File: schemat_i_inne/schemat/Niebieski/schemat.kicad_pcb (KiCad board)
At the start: 2 copper layers, 195.6 x 86.4 mm, 34 parts, among them J1 Hole1, J2 Hole2, J3 Hole3, J4 Hole4, J5 RJ45, J6 Conn_01x01_Male, J7 Conn_01x01_Male, SW1 SW_DIP_x01, SW2 Left, SW3 Up, SW4 Down, SW5 Right, SW6 Jump, SW7 Punch, U1 ATmega32A-AU, U2 L7805, U3 WG12864B-STBL, U4 LF33_TO252, U5 SN74LS07, U6 SD, Y1 16Mhz

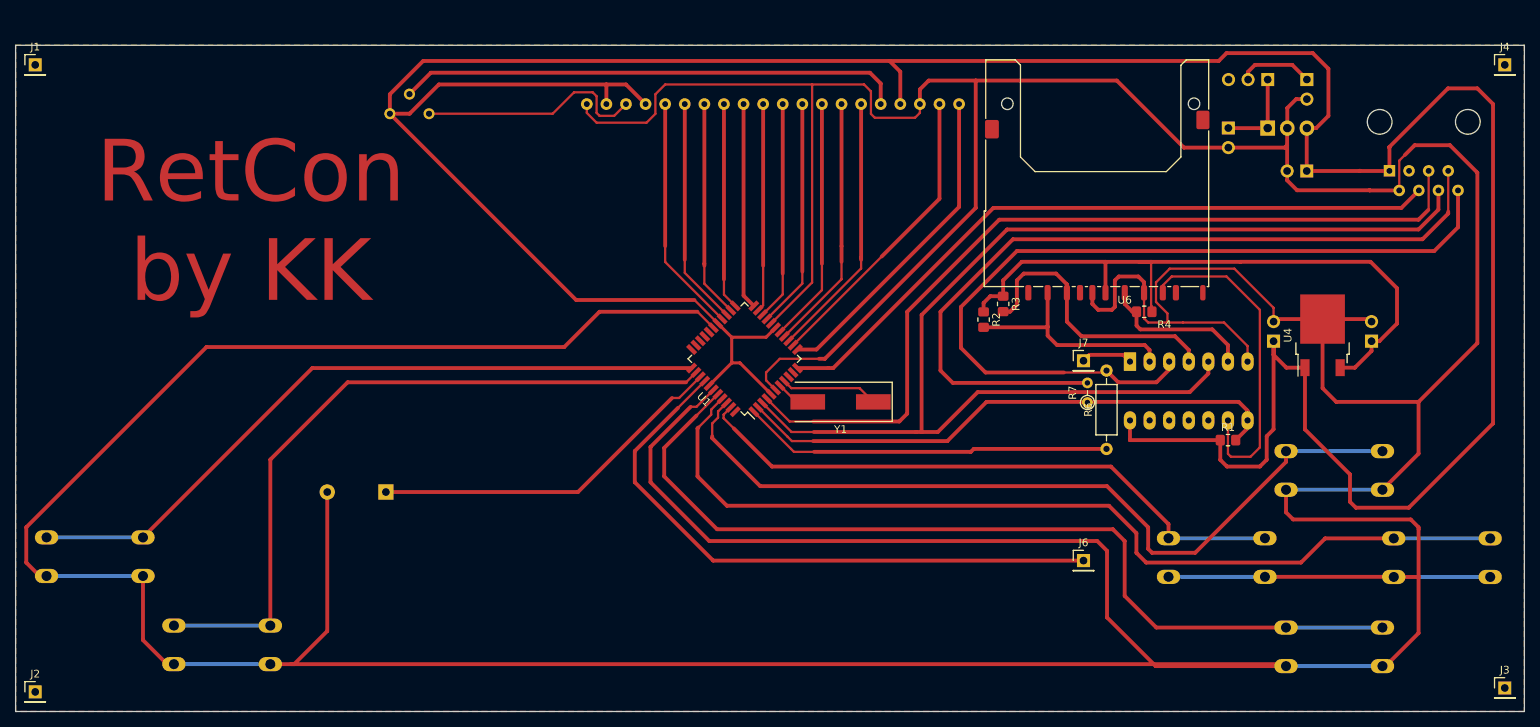
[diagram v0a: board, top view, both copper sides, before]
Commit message: new version of schema and board
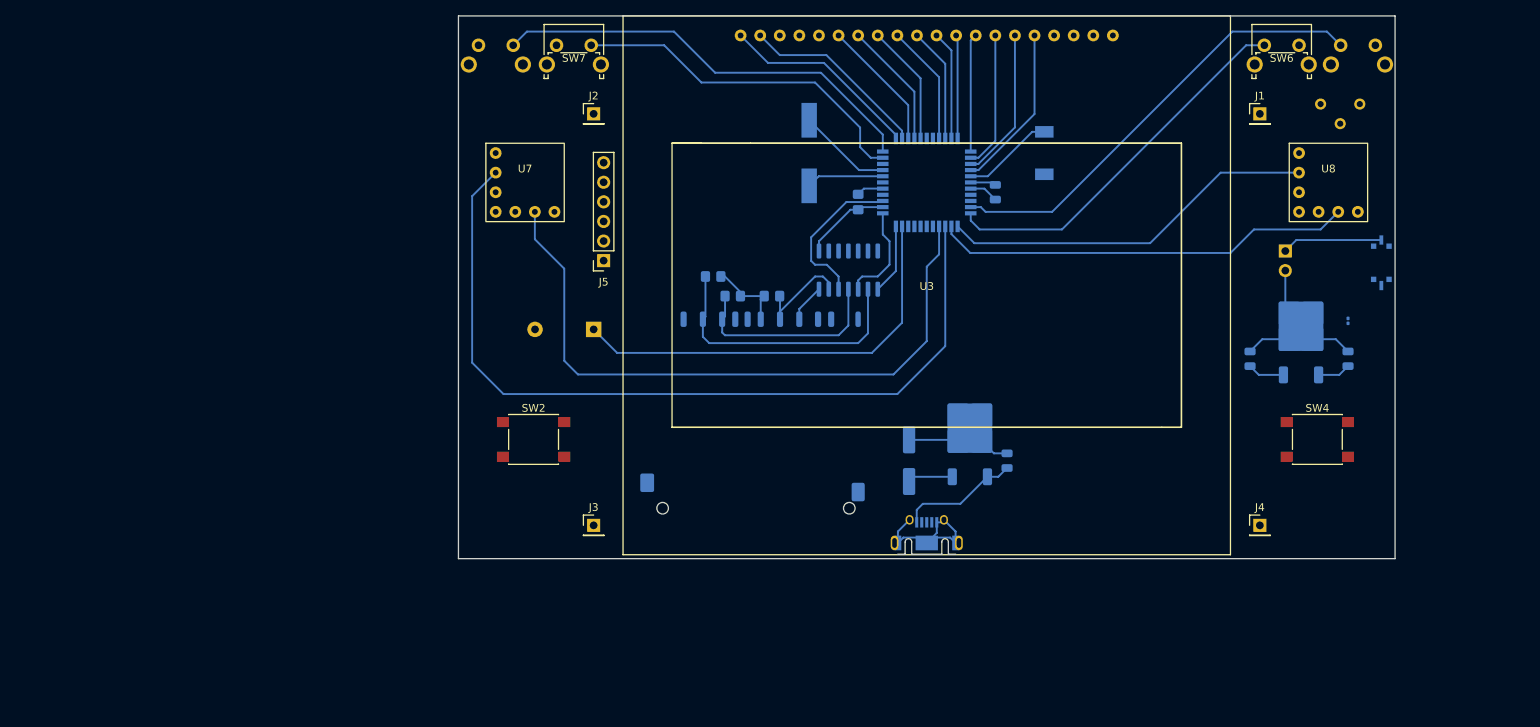
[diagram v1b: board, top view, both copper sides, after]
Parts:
- removed J7: Conn_01x01_Male, Connector_PinHeader_2.54mm:PinHeader_1x01_P2.54mm_Vertical
- removed R6: 0R, Resistor_THT:R_Axial_DIN0207_L6.3mm_D2.5mm_P10.16mm_Horizontal
- removed R7: 0R, Resistor_THT:R_Axial_DIN0204_L3.6mm_D1.6mm_P2.54mm_Vertical
- added C5: 100N, Capacitor_SMD:C_0805_2012Metric, B.Cu at (172.7, 72.4)
- added D1: D, Diode_SMD:D_0201_0603Metric, B.Cu at (218.4, 89.1)
- added L1: 10uH, Inductor_SMD:L_6.3x6.3_H3, B.Cu at (179.1, 67.3)
- added U7: ~, joystick:joystickTHT, F.Cu at (111.8, 71.1)
- added U8: ~, joystick:joystickTHT, F.Cu at (215.9, 71.1)
- BT1: footprint Connector_PinHeader_2.54mm:PinHeader_1x02_P2.54mm_Vertical -> Connector_PinSocket_2.54mm:PinSocket_1x02_P2.54mm_Vertical
- C1, C2, C3: footprint Connector_PinHeader_2.54mm:PinHeader_1x02_P2.54mm_Vertical -> Capacitor_SMD:C_0805_2012Metric
- C4: footprint Connector_PinHeader_2.54mm:PinHeader_1x02_P2.54mm_Vertical -> Capacitor_SMD:CP_Elec_6.3x5.4_Nichicon
- J5: value RJ45 -> programming port; footprint Connector_RJ:RJ45_Amphenol_54602-x08_Horizontal -> Connector_PinSocket_2.54mm:PinSocket_1x06_P2.54mm_Vertical; moved to F.Cu
- J6: value Conn_01x01_Male -> USB_B_Micro; footprint Connector_PinHeader_2.54mm:PinHeader_1x01_P2.54mm_Vertical -> Connector_USB:USB_Micro-AB_Molex_47590-0001; moved to B.Cu
- R1, R2, R3, R4, U4, U6, Y1: moved to B.Cu
- SW1: footprint Connector_PinHeader_2.54mm:PinHeader_1x03_P2.54mm_Vertical -> Button_Switch_SMD:SW_DIP_SPSTx01_Slide_Copal_CVS-01xB_W5.9mm_P1mm
- SW2: value Left -> Home; footprint Button_Switch_THT:SW_PUSH-12mm -> Button_Switch_SMD:SW_Push_1P1T_NO_6x6mm_H9.5mm; moved to F.Cu
- SW3: value Up -> triggerR; footprint Button_Switch_THT:SW_PUSH-12mm -> Button_Switch_THT:SW_Tactile_SPST_Angled_PTS645Vx31-2LFS
- SW4: value Down -> Select; footprint Button_Switch_THT:SW_PUSH-12mm -> Button_Switch_SMD:SW_Push_1P1T_NO_6x6mm_H9.5mm; moved to F.Cu
- SW5: value Right -> triggerL; footprint Button_Switch_THT:SW_PUSH-12mm -> Button_Switch_THT:SW_Tactile_SPST_Angled_PTS645Vx31-2LFS
- SW6: value Jump -> BumperL; footprint Button_Switch_THT:SW_PUSH-12mm -> Button_Switch_THT:SW_Tactile_SPST_Angled_PTS645Vx31-2LFS; moved to F.Cu
- SW7: value Punch -> BumperR; footprint Button_Switch_THT:SW_PUSH-12mm -> Button_Switch_THT:SW_Tactile_SPST_Angled_PTS645Vx31-2LFS; moved to F.Cu
- U1: value ATmega32A-AU -> ATmega1284P; moved to B.Cu
- U2: footprint Package_TO_SOT_THT:TO-220-3_Vertical -> Package_TO_SOT_SMD:TO-252-2
- U3: moved to F.Cu
- U5: footprint Package_DIP:DIP-14_W7.62mm_LongPads -> Package_SO:SO-14_3.9x8.65mm_P1.27mm
- moved J1 158.9 mm to (207.0, 62.2)
- moved SW6 149.2 mm to (207.6, 53.3), turned to 0 degrees
- moved SW5 141.9 mm to (110.2, 53.3)
- moved J3 120.0 mm to (120.7, 115.6)
- moved RV1 115.6 mm to (214.9, 61.0), turned to 180 degrees
- moved J2 104.2 mm to (120.7, 62.2)
- moved J5 102.5 mm to (121.9, 81.3), turned to 180 degrees
- moved SW2 95.7 mm to (112.9, 104.4), turned to 0 degrees
- moved SW7 83.3 mm to (115.8, 53.3), turned to 0 degrees
- moved J4 67.6 mm to (207.0, 115.6)
- moved C4 61.9 mm to (161.5, 107.2), turned to 90 degrees
- moved R1 57.0 mm to (154.9, 73.7), turned to -90 degrees
- moved U6 53.0 mm to (141.7, 101.4)
- moved SW3 52.6 mm to (222.0, 53.3)
- moved R4 48.3 mm to (143.8, 85.9), turned to 0 degrees
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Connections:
- BZ1 pad 1: Net-(BZ1-Pad1) -> Net-(BZ1--)
- C1 pad 1: Net-(C1-Pad1) -> Net-(D1-K)
- J5 pad 1: +5V -> /MOSI
- J5 pad 2: GND -> /MISO
- J5 pad 3: unconnected-(J5-Pad3) -> /SCK
- J5 pad 4: Net-(J5-Pad4) -> Net-(J5-Pin_4)
- J5 pad 5: Net-(J5-Pad5) -> +5V
- J5 pad 6: /SCK -> GND
- J6 pad 1: /CS -> +5V
- SW1 pad 1: Net-(C1-Pad1) -> Net-(D1-A)
- SW2 pad 1: Net-(SW2-Pad1) -> +5V
- SW2 pad 2: GND -> Net-(U1-PD0)
- SW3 pad 1: Net-(SW3-Pad1) -> +5V
- SW3 pad 2: GND -> Net-(U1-PA5)
- SW4 pad 1: Net-(SW4-Pad1) -> +5V
- SW4 pad 2: GND -> Net-(U1-PB2)
- SW5 pad 1: Net-(SW5-Pad1) -> Net-(U1-PD2)
- SW5 pad 2: GND -> +5V
- SW6 pad 1: Net-(SW6-Pad1) -> Net-(U1-PA4)
- SW6 pad 2: GND -> +5V
- SW7 pad 1: Net-(SW7-Pad1) -> +5V
- SW7 pad 2: GND -> Net-(U1-PD1)
- U1 pad 10: unconnected-(U1-Pad10) -> Net-(U1-PD1)
- U1 pad 11: Net-(J5-Pad4) -> Net-(U1-PD2)
- U1 pad 27: +5V -> Net-(U1-AVCC)
- U1 pad 29: unconnected-(U1-Pad29) -> Net-(U1-AREF)
- U1 pad 32: unconnected-(U1-Pad32) -> Net-(U1-PA5)
- U1 pad 33: unconnected-(U1-Pad33) -> Net-(U1-PA4)
- U1 pad 34: Net-(SW7-Pad1) -> Net-(U1-PA3)
- U1 pad 35: Net-(SW6-Pad1) -> Net-(U1-PA2)
- U1 pad 36: Net-(BZ1-Pad1) -> Net-(U1-PA1)
- U1 pad 37: /CS -> Net-(U1-PA0)
- U1 pad 4: Net-(J5-Pad5) -> Net-(J5-Pin_4)
- U1 pad 40: Net-(SW4-Pad1) -> unconnected-(U1-PB0-Pad40)
- U1 pad 41: Net-(SW5-Pad1) -> unconnected-(U1-PB1-Pad41)
- U1 pad 42: Net-(SW3-Pad1) -> Net-(U1-PB2)
- U1 pad 43: Net-(SW2-Pad1) -> Net-(BZ1--)
- U1 pad 44: unconnected-(U1-Pad44) -> /CS
- U1 pad 9: unconnected-(U1-Pad9) -> Net-(U1-PD0)
- U2 pad 1: Net-(C1-Pad1) -> Net-(D1-K)
- U5 pad 1: Net-(J7-Pad1) -> /CS
- U5 pad 3: Net-(J5-Pad8) -> /MOSI
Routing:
- net GND: track 908.8 -> 57.6 mm
- net +5V: track 425.4 -> 23.9 mm
- net /SCK: track 154.3 -> 20.3 mm
- net Net-(SW5-Pad1): track 121.6 -> 0.00 mm
- net Net-(SW4-Pad1): track 118.9 -> 0.00 mm
- net Net-(J5-Pad5): track 111.2 -> 0.00 mm
- net Net-(J5-Pad8): track 109.6 -> 0.00 mm
- net Net-(U1-PA1): track 0.00 -> 107.0 mm
- net Net-(SW3-Pad1): track 106.3 -> 0.00 mm
- net Net-(J5-Pad7): track 104.0 -> 0.00 mm
- net Net-(SW6-Pad1): track 93.9 -> 0.00 mm
- net Net-(SW7-Pad1): track 92.7 -> 0.00 mm
- net Net-(J5-Pad4): track 90.1 -> 0.00 mm
- net Net-(U1-PA0): track 0.00 -> 85.9 mm
- net Net-(SW2-Pad1): track 79.5 -> 0.00 mm
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- removed copper zone on F.Cu, net GND
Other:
- board size 195.6 x 86.4 mm -> 121.4 x 70.4 mm
- board text added: "Battery"
- board text removed: "RetCon by KK"
- board text removed: "optional- if needed"
